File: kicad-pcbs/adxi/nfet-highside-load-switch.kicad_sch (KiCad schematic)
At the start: 7 parts, among them Q19 2N7002, Q20 HY1904C2

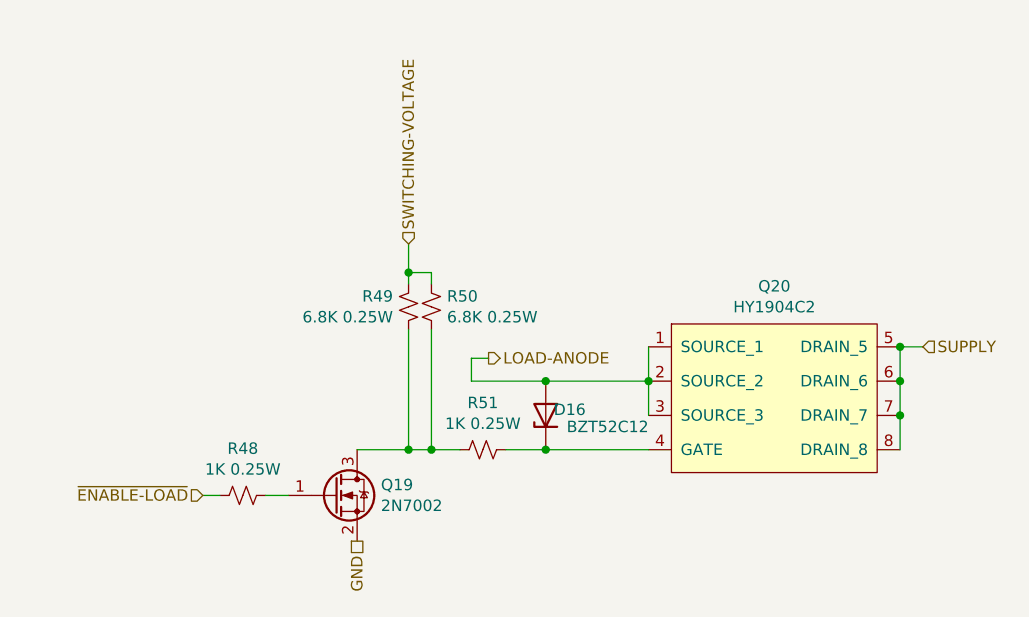
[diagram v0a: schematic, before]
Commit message: Pluggable PAs
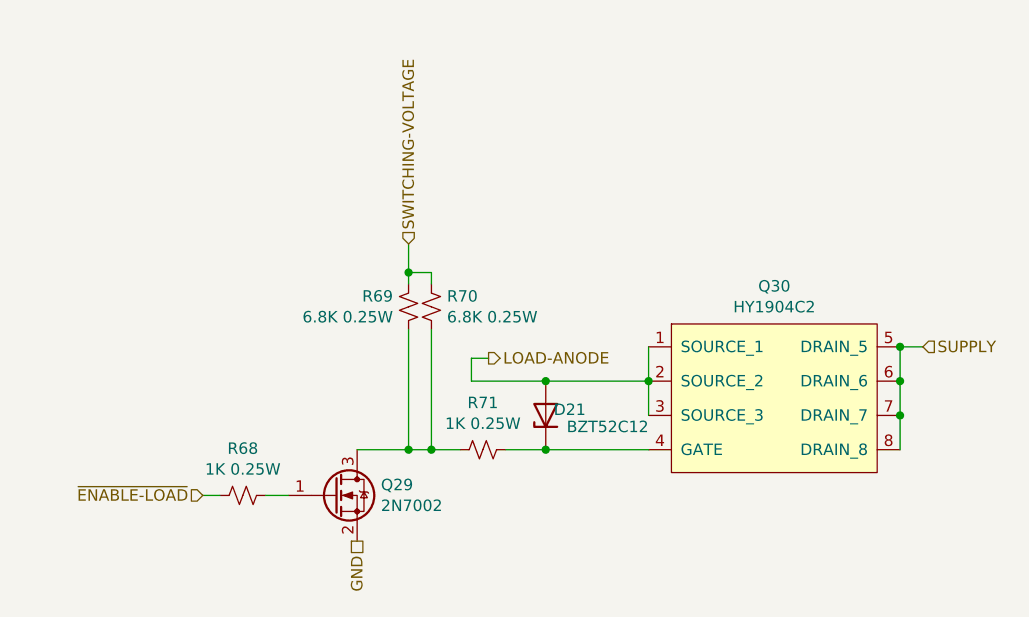
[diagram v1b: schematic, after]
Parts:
- renumbered D16 to D21, Q19 to Q29, Q20 to Q30, R48 to R68, R49 to R69, R50 to R70, R51 to R71
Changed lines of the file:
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@@
 		(on_board yes)
 		(dnp no)
-		(property "Reference" "Q20"
+		(property "Reference" "Q30"
 			(at 173.99 70.739 0)
 			(effects
@@
 		(on_board yes)
 		(dnp no)
-		(property "Reference" "D16"
+		(property "Reference" "D21"
 			(at 153.035 84.455 90)
 			(effects
@@
 		(on_board yes)
 		(dnp no)
-		(property "Reference" "R48"
+		(property "Reference" "R68"
 			(at 114.935 88.773 90)
 			(effects
@@
 		(on_board yes)
 		(dnp no)
-		(property "Reference" "Q19"
+		(property "Reference" "Q29"
 			(at 130.2766 92.8116 0)
 			(effects
@@
 		(on_board yes)
 		(dnp no)
-		(property "Reference" "R50"
+		(property "Reference" "R70"
 			(at 137.6172 71.8566 0)
 			(effects
@@
 		(on_board yes)
 		(dnp no)
-		(property "Reference" "R49"
+		(property "Reference" "R69"
 			(at 131.6228 71.8566 0)
 			(effects
@@
 		(on_board yes)
 		(dnp no)
-		(property "Reference" "R51"
+		(property "Reference" "R71"
 			(at 141.605 83.693 90)
 			(effects
